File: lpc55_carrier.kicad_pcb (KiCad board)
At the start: 4 copper layers, 51.4 x 37.1 mm, 58 parts, among them J101 Conn_2Rows-51Pins, U101 LPC55S28JBD64, Y101 16MHz 18pF, Y102 32.768kHz 12.5pF

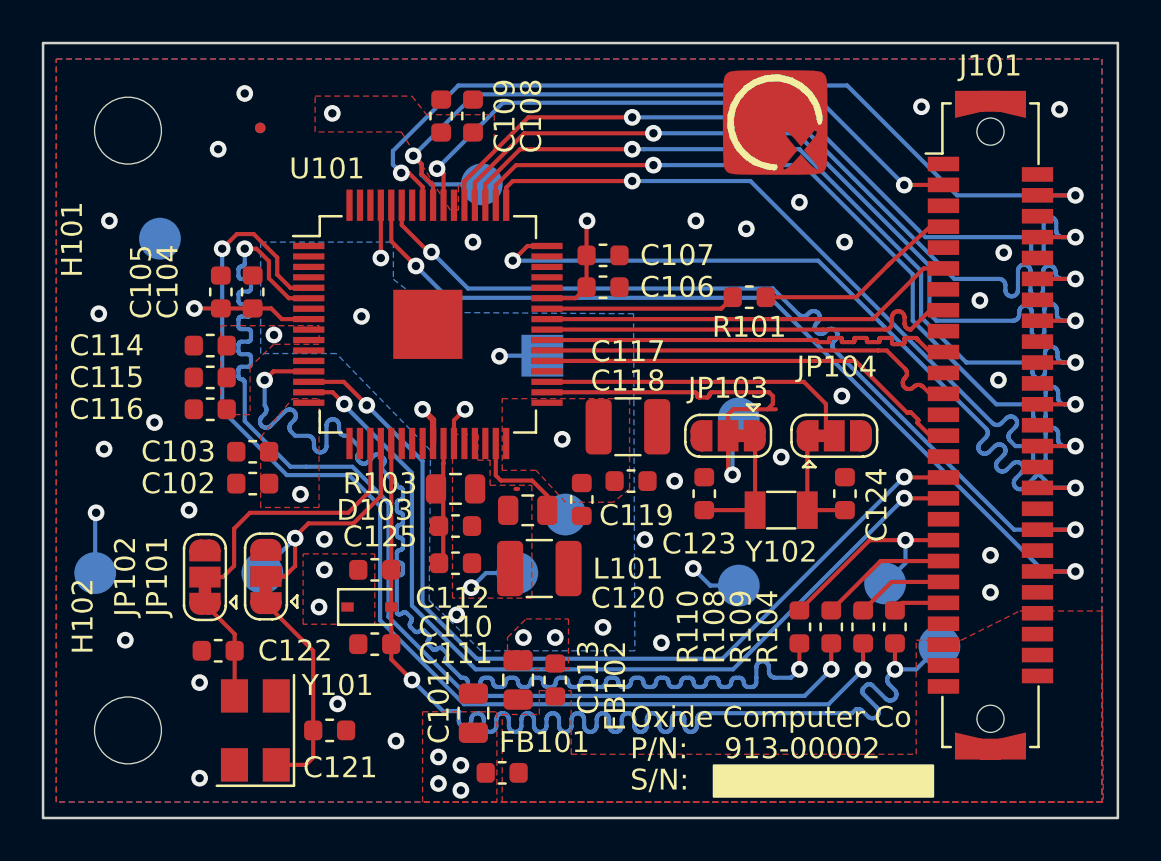
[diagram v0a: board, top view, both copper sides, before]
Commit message: lpc55_carrier: shrink silkscreen to 0.75mm width and height
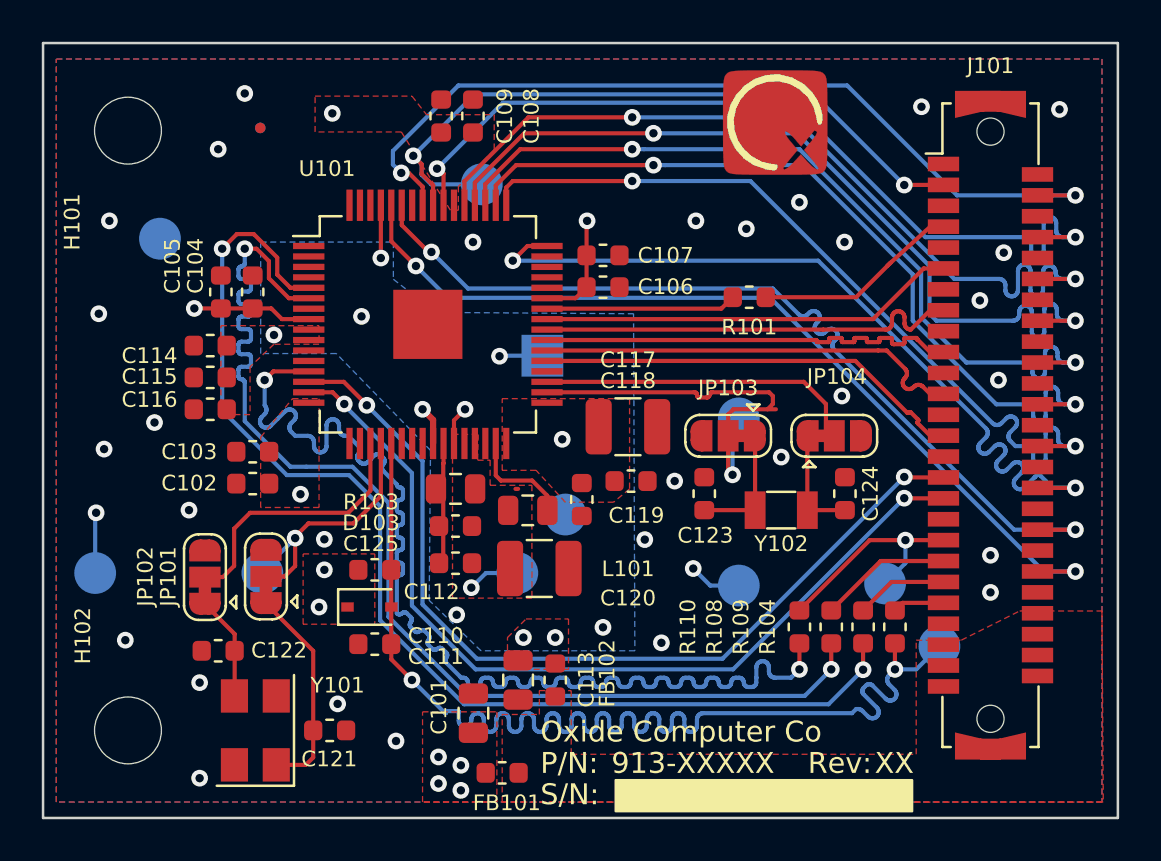
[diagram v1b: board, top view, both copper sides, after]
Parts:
- removed the G*** at (96.1, 83.8)
- added G***: 913-XXXXX, grumpy:Oxide_Board_Identifier_18x5mm, F.Cu at (91.8, 84.5)
